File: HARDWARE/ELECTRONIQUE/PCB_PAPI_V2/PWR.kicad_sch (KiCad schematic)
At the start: 36 parts, among them IC1 LMR51625YFDDCR, IC2 LDO40LPU33RY, IC3 LDO40LPU33RY, Q1 STR2N2VH5

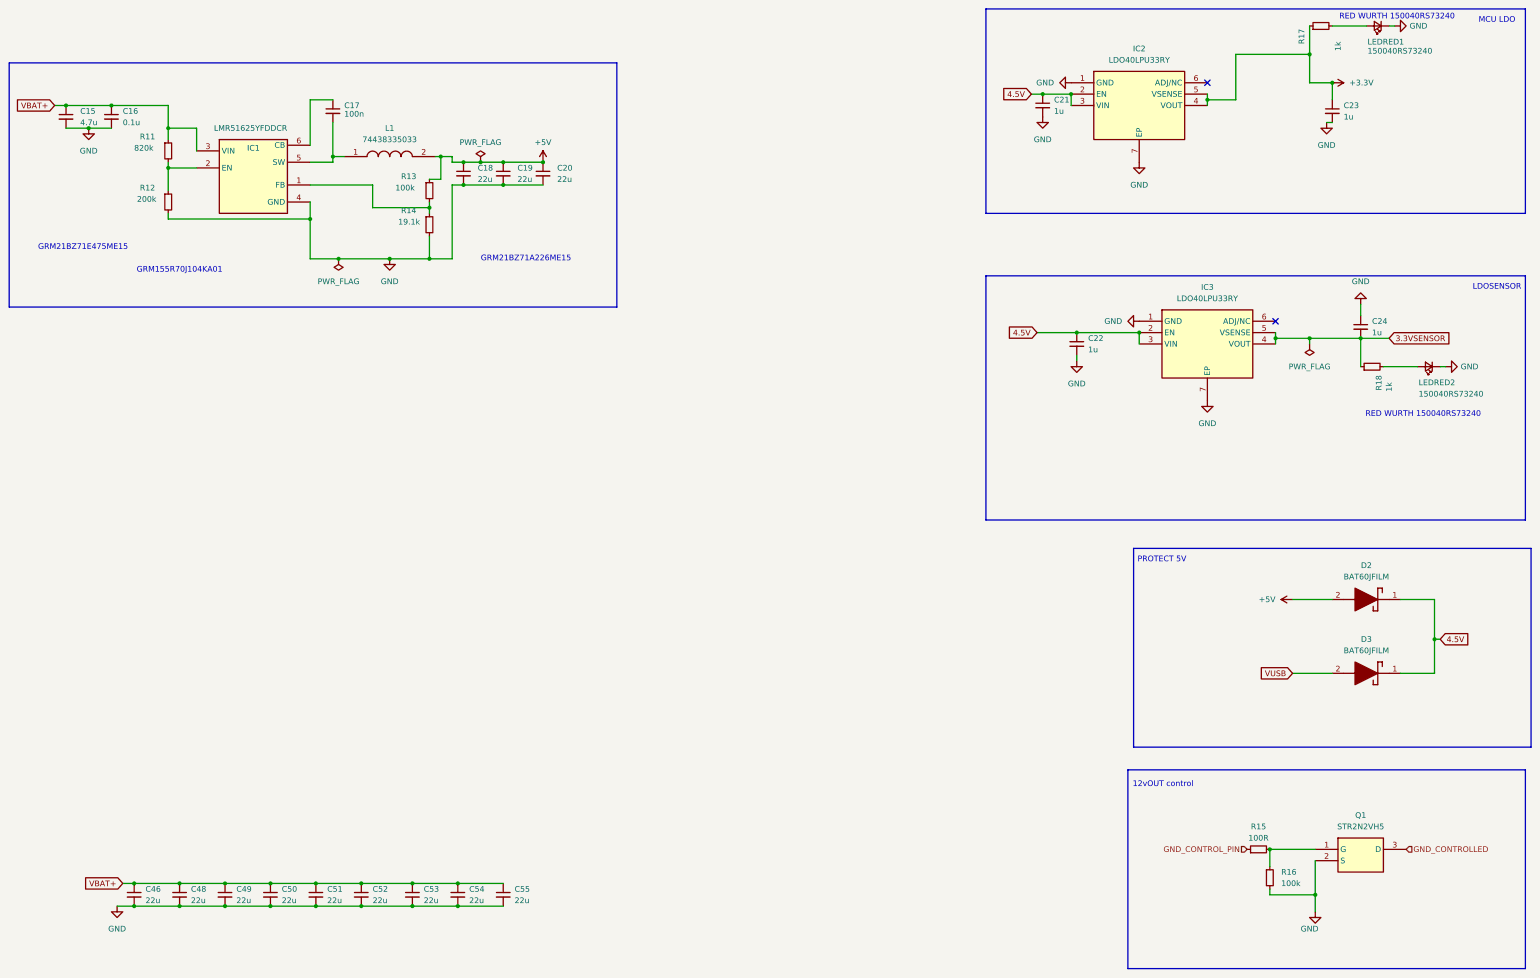
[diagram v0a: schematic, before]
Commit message: up
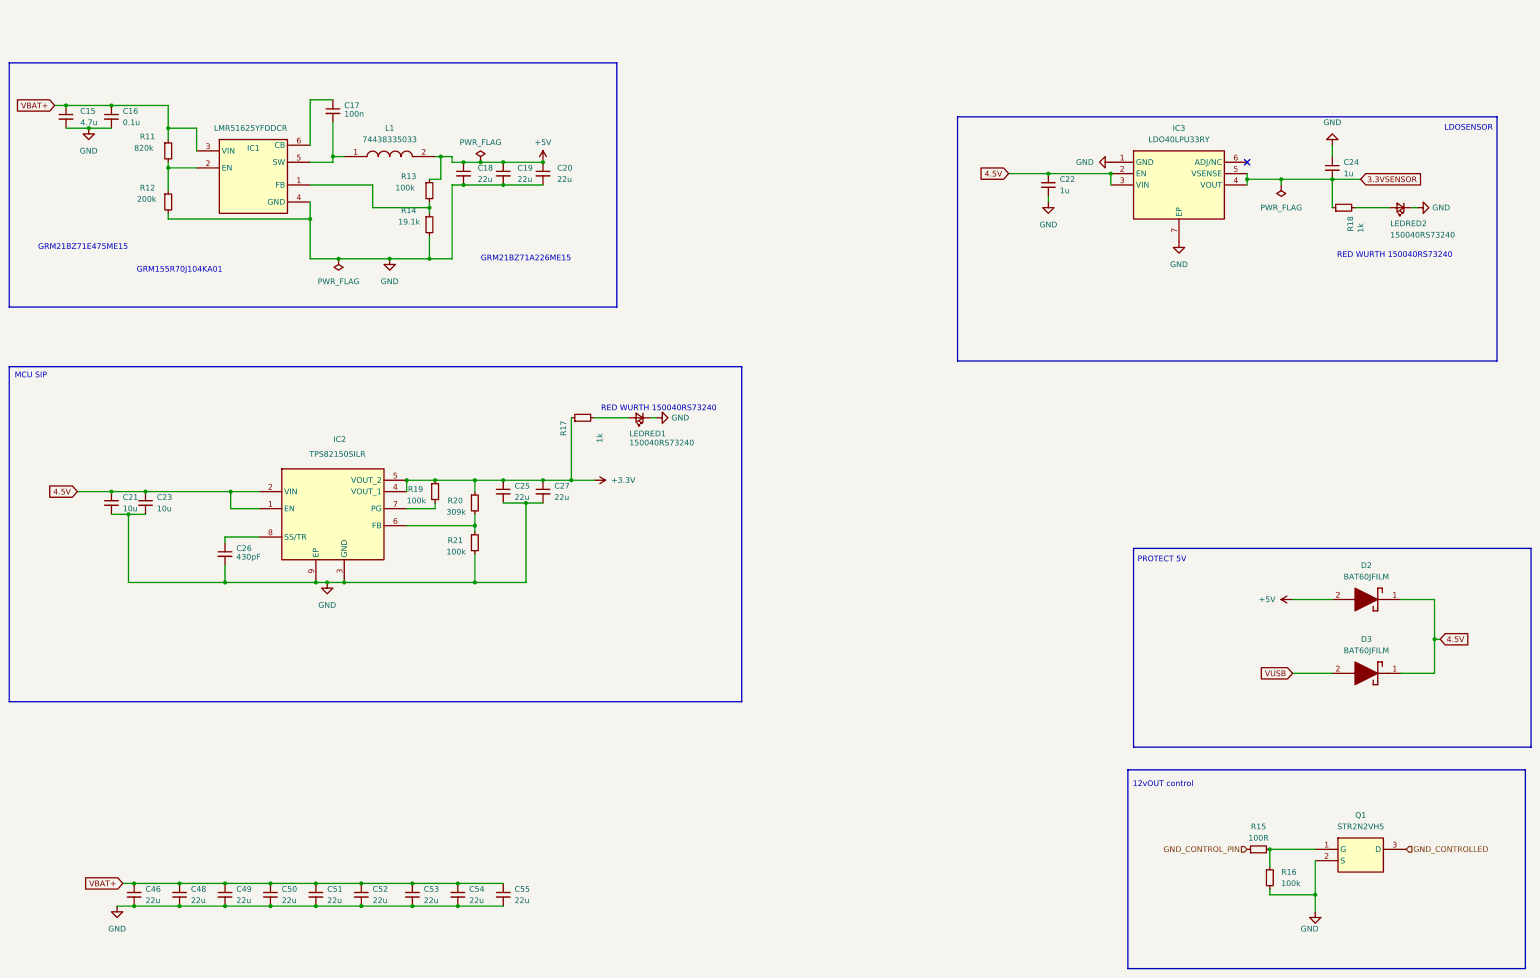
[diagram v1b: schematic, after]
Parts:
- removed IC2: LDO40LPU33RY, samacsys:SON95P300X300X90-7N-D, symbol ldo40puryy:LDO40LPU33RY
- added C25, C27: 22u, Capacitor_SMD:C_0603_1608Metric, symbol Device:C_Small
- added C26: 430pF, Capacitor_SMD:C_0201_0603Metric, symbol Device:C_Small
- added IC2: TPS82150SILR, samacsys2:TPS82130SILT, symbol samacsys:TPS82150SILR
- added R19, R21: 100k, Resistor_SMD:R_0201_0603Metric, symbol Device:R_Small
- added R20: 309k, Resistor_SMD:R_0201_0603Metric, symbol Device:R_Small
- C21, C23: value 1u -> 10u; footprint Capacitor_SMD:C_0402_1005Metric -> Capacitor_SMD:C_0603_1608Metric
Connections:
- net +3.3V: now also C25.1, C27.1, IC2.4 (VOUT_1), IC2.5 (VOUT_2), R19.1, R20.1; no longer C23.1
- net 4.5V: now also C23.1, IC2.1 (EN), IC2.2 (VIN)
- net GND: now also C25.2, C26.2, C27.2, IC2.3 (GND), IC2.9 (EP), R21.2
- new net: IC2.6 (FB), R20.2, R21.1
- new net: C26.1, IC2.8 (SS/TR)
- new net: IC2.7 (PG), R19.2
- no-connect marks 2 -> 1
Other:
- note added: "MCU SIP"
- note removed: "MCU LDO"
- moved on the sheet: C21, C22, C24, IC3, LEDRED1, LEDRED2, R17, R18
